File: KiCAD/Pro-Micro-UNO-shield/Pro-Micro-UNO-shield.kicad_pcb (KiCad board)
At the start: 2 copper layers, 68.6 x 53 mm, 58 parts, among them J1 Arduino_pro_micro, J15 Debug LED enable, J2 Arduino UNO, J3 Conn_01x10_Male, J5 Arduino_pro_micro WIDE, J6 Conn_01x10_Male, J7 Conn_01x02_Male

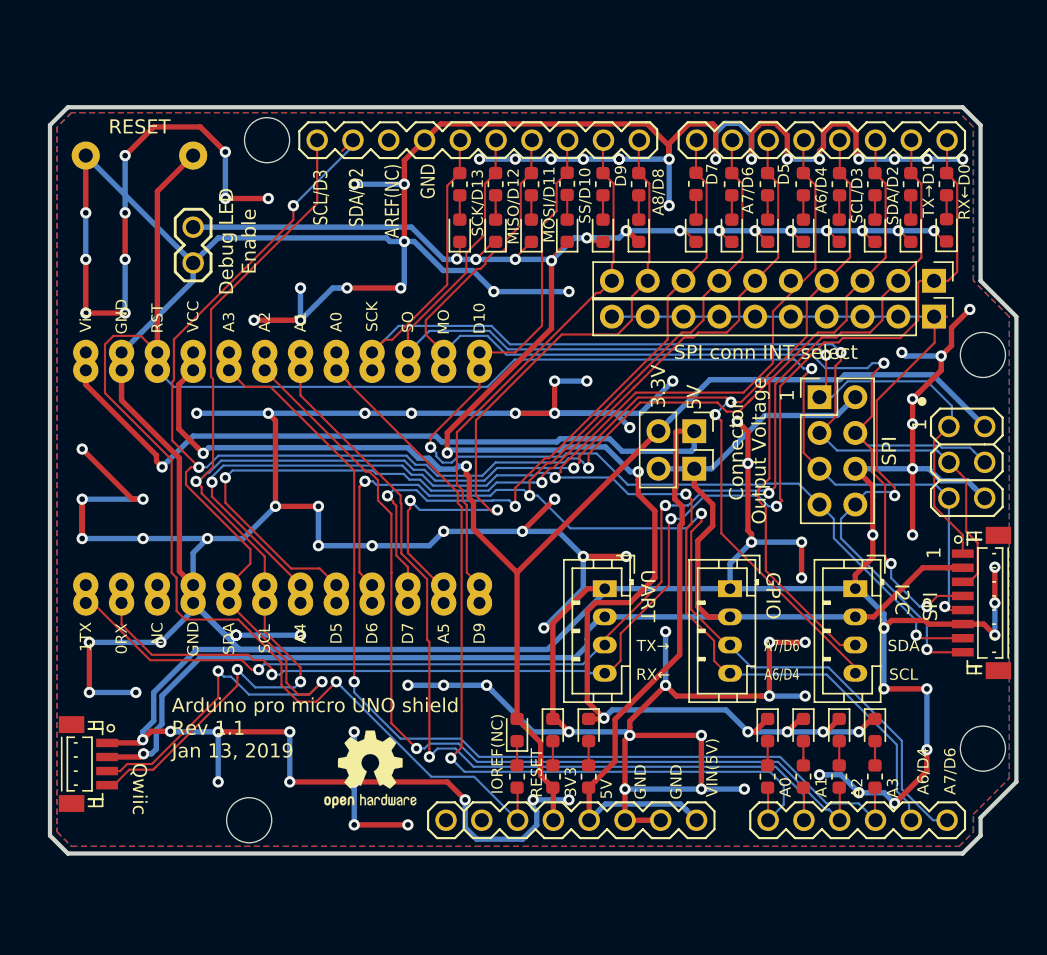
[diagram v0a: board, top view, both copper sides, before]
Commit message: Pro Micro UNO shield v2.0 (Diag shield)
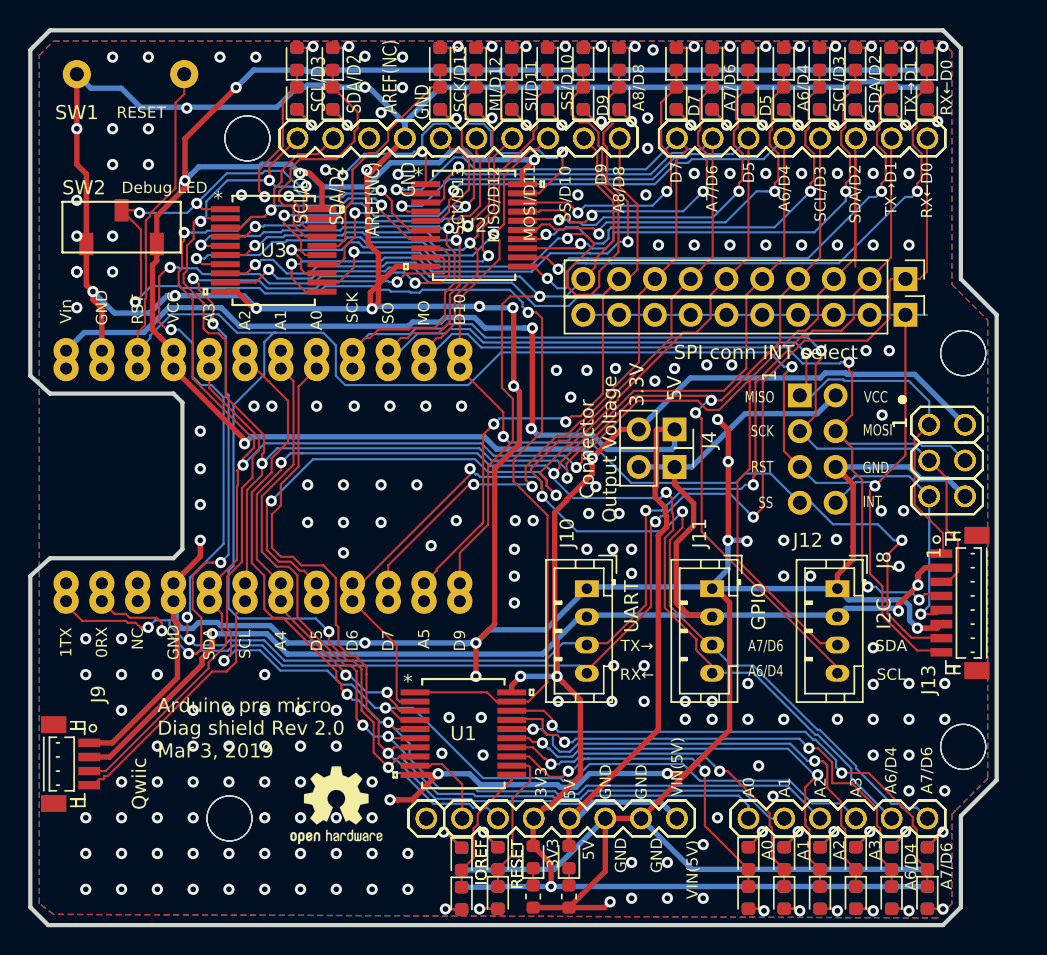
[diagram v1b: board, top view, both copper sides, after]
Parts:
- removed Connector output Voltage: Conn_01x02_Male, KiCAD footprints:PinHeader_1x02_P2.54mm_Vertical
- removed Grove GPIO: Grove GPIO, library:JST_PH_B4B-PH-K_04x2.00mm_Straight
- removed Grove I2C: Grove I2C, library:JST_PH_B4B-PH-K_04x2.00mm_Straight
- removed Grove UART: Grove UART, library:JST_PH_B4B-PH-K_04x2.00mm_Straight
- removed J15: Debug LED enable, freetronics_footprints:1X02
- removed the J2 at (120.8, 166.5)
- removed Qwiic I2C: Qwiic I2c, library:Qwiic_I2C_1.00mm_4pin
- removed RESET: Reset switch, library:push switch
- removed SPI: SPI header, KiCAD footprints:PinHeader_2x04_P2.54mm_Vertical
- removed SPI: SPI connector, library:JST_SH_BM08B-SRSS-TB_08x1.00mm_Straight
- added D22: BLUE, LED_SMD:LED_0603_1608Metric, F.Cu at (156.0, 110.0)
- added D23: BLUE, LED_SMD:LED_0603_1608Metric, F.Cu at (158.5, 110.0)
- added D24: BLUE, LED_SMD:LED_0603_1608Metric, F.Cu at (161.0, 110.0)
- added D25: PWR, LED_SMD:LED_0603_1608Metric, F.Cu at (154.9, 166.6)
- added D26: RED, LED_SMD:LED_0603_1608Metric, F.Cu at (182.9, 166.7)
- added D27: RED, LED_SMD:LED_0603_1608Metric, F.Cu at (180.4, 166.7)
- added D28: RED, LED_SMD:LED_0603_1608Metric, F.Cu at (177.8, 166.7)
- added D29: RED, LED_SMD:LED_0603_1608Metric, F.Cu at (175.3, 166.7)
- added D30: RED, LED_SMD:LED_0603_1608Metric, F.Cu at (172.8, 166.7)
- added D31: RED, LED_SMD:LED_0603_1608Metric, F.Cu at (170.2, 166.7)
- added D32: RED, LED_SMD:LED_0603_1608Metric, F.Cu at (152.4, 166.7)
- added D33: RED, LED_SMD:LED_0603_1608Metric, F.Cu at (149.9, 166.8)
- added D34: RED, LED_SMD:LED_0603_1608Metric, F.Cu at (165.1, 112.8)
- added D35: RED, LED_SMD:LED_0603_1608Metric, F.Cu at (167.6, 112.8)
- added D36: RED, LED_SMD:LED_0603_1608Metric, F.Cu at (170.2, 112.8)
- added D37: RED, LED_SMD:LED_0603_1608Metric, F.Cu at (172.7, 112.8)
- added D38: RED, LED_SMD:LED_0603_1608Metric, F.Cu at (175.3, 112.8)
- added D39: RED, LED_SMD:LED_0603_1608Metric, F.Cu at (177.8, 112.8)
- added D40: RED, LED_SMD:LED_0603_1608Metric, F.Cu at (180.3, 112.8)
- added D41: RED, LED_SMD:LED_0603_1608Metric, F.Cu at (182.9, 112.8)
- added D42: RED, LED_SMD:LED_0603_1608Metric, F.Cu at (138.2, 112.8)
- added D43: RED, LED_SMD:LED_0603_1608Metric, F.Cu at (140.7, 112.8)
- added D44: RED, LED_SMD:LED_0603_1608Metric, F.Cu at (148.3, 112.8)
- added D45: RED, LED_SMD:LED_0603_1608Metric, F.Cu at (150.9, 112.8)
- added D46: RED, LED_SMD:LED_0603_1608Metric, F.Cu at (153.4, 112.8)
- added D47: RED, LED_SMD:LED_0603_1608Metric, F.Cu at (156.0, 112.8)
- added D48: RED, LED_SMD:LED_0603_1608Metric, F.Cu at (158.5, 112.8)
- added D49: RED, LED_SMD:LED_0603_1608Metric, F.Cu at (161.0, 112.8)
- added D50: PWR, LED_SMD:LED_0603_1608Metric, F.Cu at (157.5, 166.6)
- added J10: Grove UART, library:JST_PH_B4B-PH-K_04x2.00mm_Straight, F.Cu at (158.8, 147.6)
- added J11: Grove GPIO, library:JST_PH_B4B-PH-K_04x2.00mm_Straight, F.Cu at (167.6, 147.6)
- added J12: SPI header, Connector_PinSocket_2.54mm:PinSocket_2x04_P2.54mm_Vertical, B.Cu at (173.9, 133.9)
- added J13: SPI connector, library:JST_SH_BM08B-SRSS-TB_08x1.00mm_Straight, F.Cu at (185.2, 148.6)
- added J2 (x2): Arduino UNO, library:Arduino_Shield, F.Cu at (119.4, 166.4)
- added J4: Conn_01x02_Male, Connector_PinSocket_2.54mm:PinSocket_1x02_P2.54mm_Vertical, F.Cu at (165.0, 136.3)
- added J8: Grove I2C, library:JST_PH_B4B-PH-K_04x2.00mm_Straight, F.Cu at (176.5, 147.6)
- added J9: Qwiic I2c, library:Qwiic_I2C_1.00mm_4pin, F.Cu at (122.2, 160.0)
- added R22: 220R, Resistor_SMD:R_0603_1608Metric, B.Cu at (156.0, 110.0)
- added R23: 220R, Resistor_SMD:R_0603_1608Metric, B.Cu at (158.5, 110.0)
- added R24: 220R, Resistor_SMD:R_0603_1608Metric, B.Cu at (161.0, 110.0)
- added R25: 220R, Resistor_SMD:R_0603_1608Metric, F.Cu at (154.9, 169.4)
- added R26: 220R, Resistor_SMD:R_0603_1608Metric, B.Cu at (182.9, 166.7)
- added R27: 220R, Resistor_SMD:R_0603_1608Metric, B.Cu at (180.4, 166.7)
- added R28: 220R, Resistor_SMD:R_0603_1608Metric, B.Cu at (177.8, 166.7)
- added R29: 220R, Resistor_SMD:R_0603_1608Metric, B.Cu at (175.3, 166.7)
- added R30: 220R, Resistor_SMD:R_0603_1608Metric, B.Cu at (172.8, 166.7)
- added R31: 220R, Resistor_SMD:R_0603_1608Metric, B.Cu at (170.2, 166.7)
- added R32: 220R, Resistor_SMD:R_0603_1608Metric, B.Cu at (152.4, 166.7)
- added R33: 220R, Resistor_SMD:R_0603_1608Metric, B.Cu at (149.9, 166.8)
- added R34: 220R, Resistor_SMD:R_0603_1608Metric, B.Cu at (165.1, 112.8)
- added R35: 220R, Resistor_SMD:R_0603_1608Metric, B.Cu at (167.6, 112.8)
- added R36: 220R, Resistor_SMD:R_0603_1608Metric, B.Cu at (170.2, 112.8)
- added R37: 220R, Resistor_SMD:R_0603_1608Metric, B.Cu at (172.7, 112.8)
- added R38: 220R, Resistor_SMD:R_0603_1608Metric, B.Cu at (175.3, 112.8)
- added R39: 220R, Resistor_SMD:R_0603_1608Metric, B.Cu at (177.8, 112.8)
- added R40: 220R, Resistor_SMD:R_0603_1608Metric, B.Cu at (180.3, 112.8)
- added R41: 220R, Resistor_SMD:R_0603_1608Metric, B.Cu at (182.9, 112.8)
- added R42: 220R, Resistor_SMD:R_0603_1608Metric, B.Cu at (138.2, 112.8)
- added R43: 220R, Resistor_SMD:R_0603_1608Metric, B.Cu at (140.7, 112.8)
- added R44: 220R, Resistor_SMD:R_0603_1608Metric, B.Cu at (148.3, 112.8)
- added R45: 220R, Resistor_SMD:R_0603_1608Metric, B.Cu at (150.9, 112.8)
- added R46: 220R, Resistor_SMD:R_0603_1608Metric, B.Cu at (153.4, 112.8)
- added R47: 220R, Resistor_SMD:R_0603_1608Metric, B.Cu at (156.0, 112.8)
- added R48: 220R, Resistor_SMD:R_0603_1608Metric, B.Cu at (158.5, 112.8)
- added R49: 220R, Resistor_SMD:R_0603_1608Metric, B.Cu at (161.0, 112.8)
- added R50: 220R, Resistor_SMD:R_0603_1608Metric, F.Cu at (157.5, 169.4)
- added SW1: Reset switch, library:push switch, F.Cu at (126.4, 111.1)
- added SW2: SW_SPDT, library:mini_slide_switch, F.Cu at (125.7, 121.9)
- added U1: SN74LVC541ADBR, library:SN74LVC541ADBR, F.Cu at (150.0, 157.9)
- added U2: SN74LVC541ADBR, library:SN74LVC541ADBR, F.Cu at (150.7, 121.8)
- added U3: SN74LVC541ADBR, library:SN74LVC541ADBR, F.Cu at (136.5, 123.6)
- D1, D10, D11, D12, D13, D14, D15, D16, D17, D18, D19, D2, D20, D21, D3, D4, D5, D6, D7, D8, D9: value LED -> BLUE
- R1, R10, R11, R12, R13, R14, R15, R16, R17, R18, R19, R2, R20, R21, R3, R4, R5, R6, R7, R8, R9: value R 1K -> 220R; moved to B.Cu
- moved R17 63.8 mm to (138.2, 110.0)
- moved R18 63.8 mm to (140.7, 110.0)
- moved D17 61.2 mm to (138.2, 110.0), turned to 90 degrees
- moved D18 61.2 mm to (140.7, 110.0), turned to 90 degrees
- moved R8 58.6 mm to (149.9, 169.5)
- moved R7 56.1 mm to (152.4, 169.5)
- moved D8 55.7 mm to (149.9, 169.5), turned to 270 degrees
- moved R1 55.6 mm to (182.9, 169.5)
- moved R2 53.7 mm to (180.4, 169.5)
- moved D7 53.2 mm to (152.4, 169.5), turned to 270 degrees
- moved D1 52.6 mm to (182.9, 169.5), turned to 270 degrees
- moved R19 52.0 mm to (148.3, 110.0)
- moved R3 51.9 mm to (177.8, 169.5)
- moved R15 51.7 mm to (180.3, 110.0)
- moved R16 51.7 mm to (182.9, 110.0)
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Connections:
- D10 pad 1: Net-(D1-Pad1) -> Net-(D10-Pad1)
- D11 pad 1: Net-(D1-Pad1) -> Net-(D11-Pad1)
- D12 pad 1: Net-(D1-Pad1) -> Net-(D12-Pad1)
- D13 pad 1: Net-(D1-Pad1) -> Net-(D13-Pad1)
- D14 pad 1: Net-(D1-Pad1) -> Net-(D14-Pad1)
- D15 pad 1: Net-(D1-Pad1) -> Net-(D15-Pad1)
- D16 pad 1: Net-(D1-Pad1) -> Net-(D16-Pad1)
- D17 pad 1: Net-(D1-Pad1) -> Net-(D17-Pad1)
- D18 pad 1: Net-(D1-Pad1) -> Net-(D18-Pad1)
- D19 pad 1: Net-(D1-Pad1) -> Net-(D19-Pad1)
- D2 pad 1: Net-(D1-Pad1) -> Net-(D2-Pad1)
- D20 pad 1: GND -> Net-(D20-Pad1)
- D21 pad 2: 3.3V -> Net-(D21-Pad2)
- D3 pad 1: Net-(D1-Pad1) -> Net-(D28-Pad2)
- D4 pad 1: Net-(D1-Pad1) -> Net-(D29-Pad2)
- D5 pad 1: Net-(D1-Pad1) -> Net-(D30-Pad2)
- D6 pad 1: Net-(D1-Pad1) -> Net-(D31-Pad2)
- D7 pad 1: Net-(D1-Pad1) -> Net-(D32-Pad2)
- D8 pad 1: Net-(D1-Pad1) -> Net-(D33-Pad2)
- D9 pad 1: Net-(D1-Pad1) -> Net-(D34-Pad2)
- R1 pad 2: D9 -> 3.3V
- R10 pad 2: TX -> 3.3V
- R11 pad 2: D10/SS -> 3.3V
- R12 pad 2: MOSI -> 3.3V
- R13 pad 2: MISO -> 3.3V
- R14 pad 2: SCK -> 3.3V
- R15 pad 2: A0 -> 3.3V
- R16 pad 2: A1 -> 3.3V
- R17 pad 2: A2 -> 3.3V
- R18 pad 2: A3 -> 3.3V
- R19 pad 2: 5V -> 3.3V
- R2 pad 2: D8/A8 -> 3.3V
- R21 pad 1: Net-(D21-Pad1) -> Net-(D21-Pad2)
- R21 pad 2: RESET -> 3.3V
- R3 pad 2: D7 -> 3.3V
- R4 pad 2: D6/A7 -> 3.3V
- R5 pad 2: D5 -> 3.3V
- R6 pad 2: D4/A6 -> 3.3V
- R7 pad 2: SCL -> 3.3V
- R8 pad 2: SDA -> 3.3V
- R9 pad 2: RX -> 3.3V
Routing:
- net GND: track 661.9 -> 379.6 mm, vias 120 -> 202
- net 3.3V: track 96.1 -> 241.9 mm, vias 2 -> 9
- net /debug_led/OE: track 0.00 -> 128.4 mm, vias 0 -> 8
- net Net-(D1-Pad1): track 153.1 -> 37.7 mm, vias 21 -> 2
- net TX: track 91.9 -> 147.0 mm, vias 3 -> 8
- net RX: track 96.4 -> 147.6 mm, vias 3 -> 8
- net Net-(D23-Pad1): track 0.00 -> 47.1 mm, vias 0 -> 2
- net Net-(D24-Pad1): track 0.00 -> 42.5 mm, vias 0 -> 2
- net Net-(D16-Pad1): track 0.00 -> 41.5 mm, vias 0 -> 2
- net Net-(D15-Pad1): track 0.00 -> 37.5 mm, vias 0 -> 2
- net Net-(D2-Pad1): track 0.00 -> 36.1 mm, vias 0 -> 2
- net Net-(D14-Pad1): track 0.00 -> 34.8 mm, vias 0 -> 2
- net Net-(D28-Pad2): track 0.00 -> 33.8 mm, vias 0 -> 2
- net Net-(D22-Pad1): track 0.00 -> 33.4 mm, vias 0 -> 2
- net Net-(D13-Pad1): track 0.00 -> 32.5 mm, vias 0 -> 2
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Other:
- board size 68.6 x 53 mm -> 68.6 x 63.5 mm
- board text added: "Arduino pro micro Diag shield Rev 2.0 Mar 3, 2019"
- board text added: "Debug LED"
- board text added: "GND"
- board text added: "INT"
- board text added: "MISO"
- board text added: "MOSI"
- board text added: "RESET"
- board text added: "RST"
- board text added: "SCK"
- board text added: "SS"
- board text added: "VCC"
- board text removed: "Arduino pro micro UNO shield Rev 1.1 Jan 13, 2019"
- board text removed: "Debug LED Enable"
